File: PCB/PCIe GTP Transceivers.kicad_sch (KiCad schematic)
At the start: 1 part, among them U1 XC7A50T-FGG484

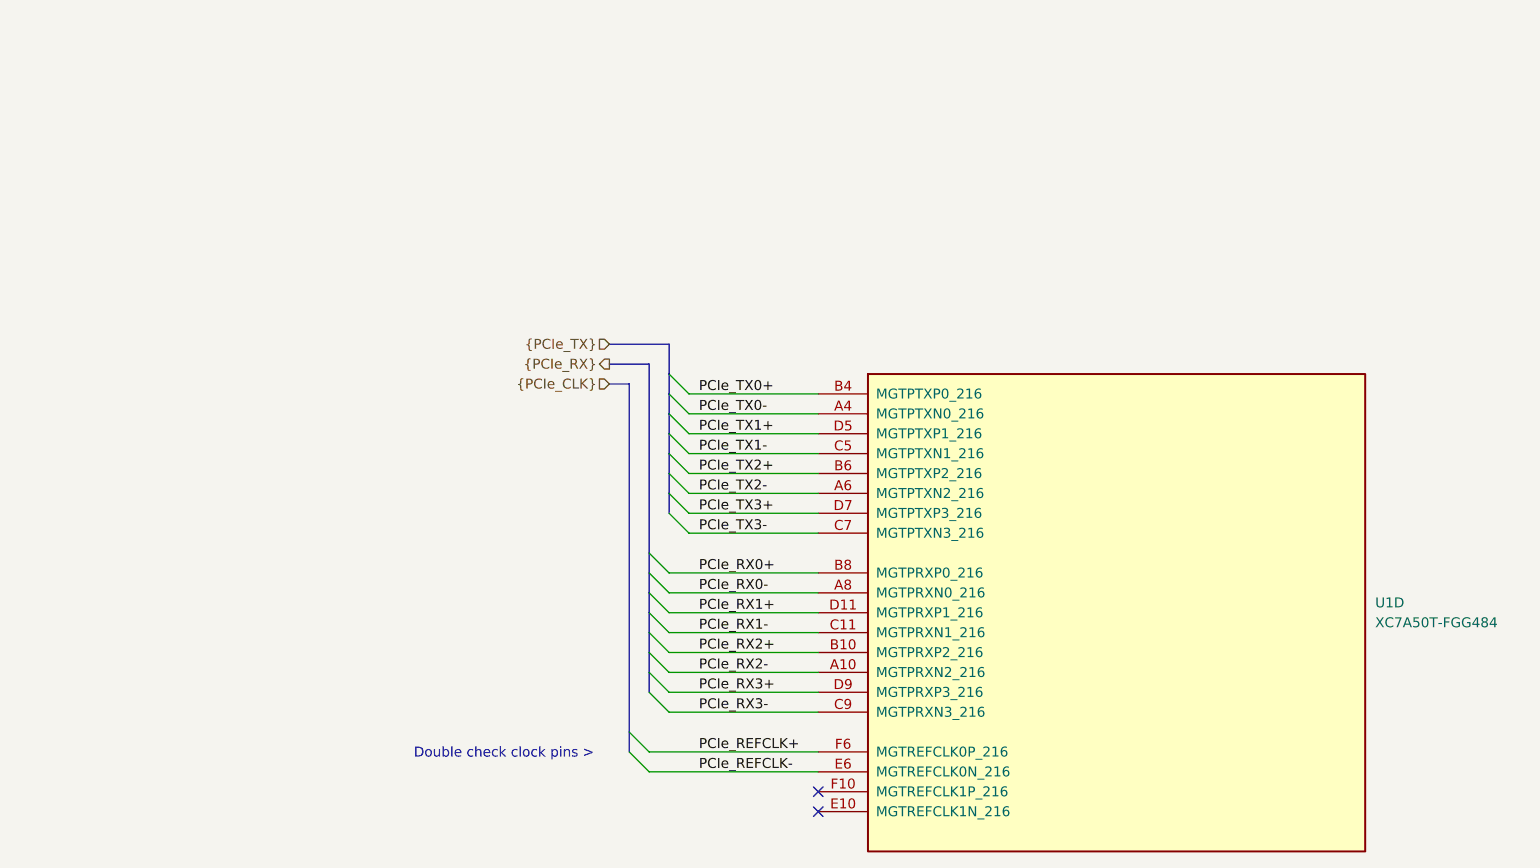
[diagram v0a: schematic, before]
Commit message: cleaning up the schematic even more, starting on HDMI
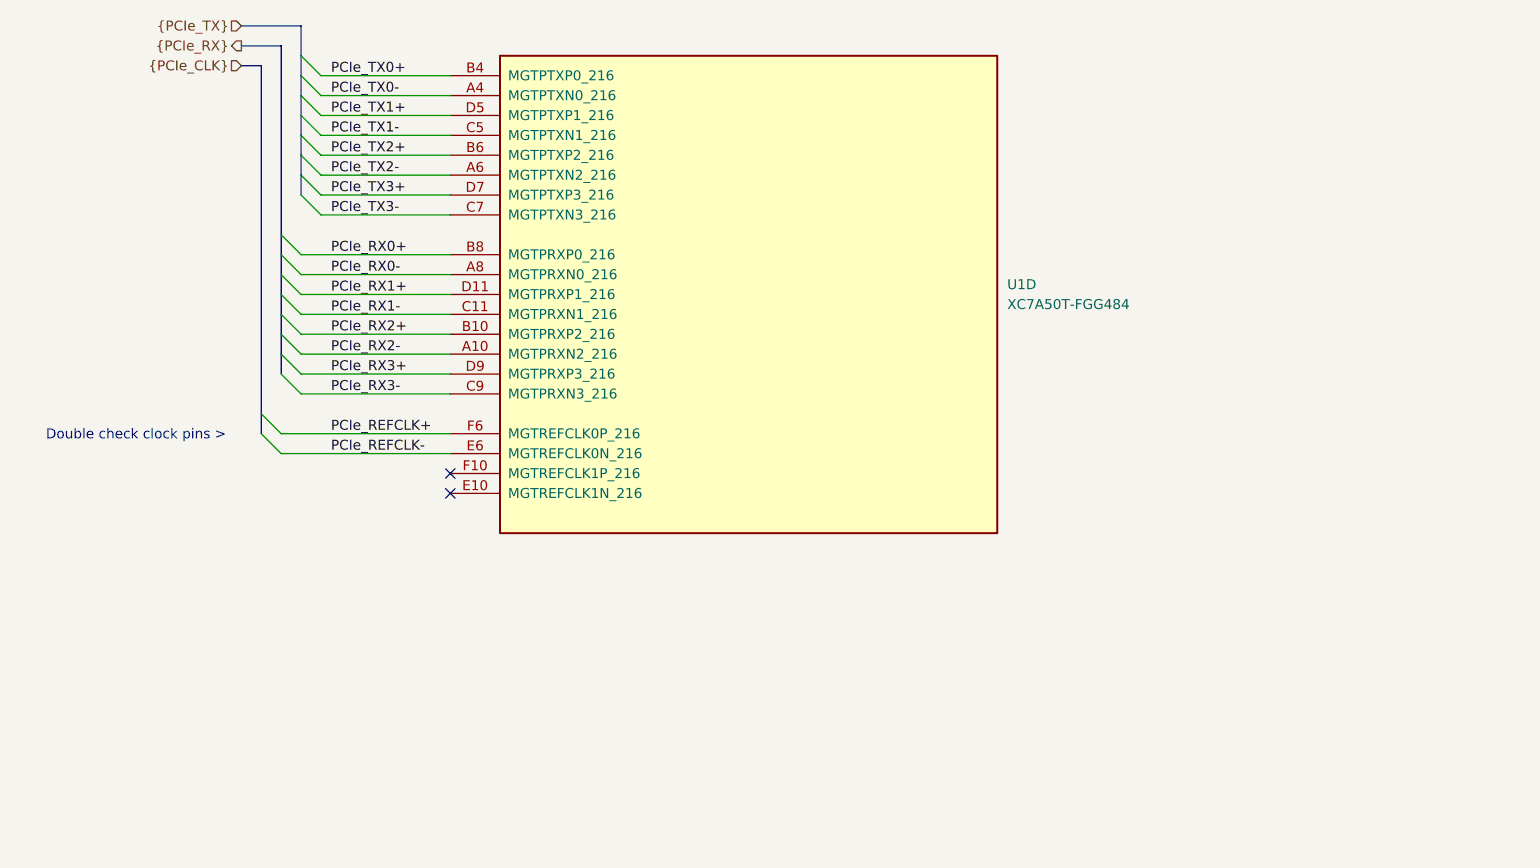
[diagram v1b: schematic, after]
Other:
- moved on the sheet: U1D
